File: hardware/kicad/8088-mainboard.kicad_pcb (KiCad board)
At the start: 2 copper layers, 170 x 125 mm, 45 parts, among them J1 Conn_01x10, J2 Exp0, J3 Exp1, J4 POWER 5v, J5 Ext CLK, Q1 NDP6020P, SW1 Reset, SW2 SW_DIP_x02, U1 8088_Min_Mode, U2 74LS373, U3 74LS373, U4 74LS245, U5 8284, U6 74LS138, U7 74LS138, U8 28C256, U9 HM62256BLP, Y1 14.31818 MHz

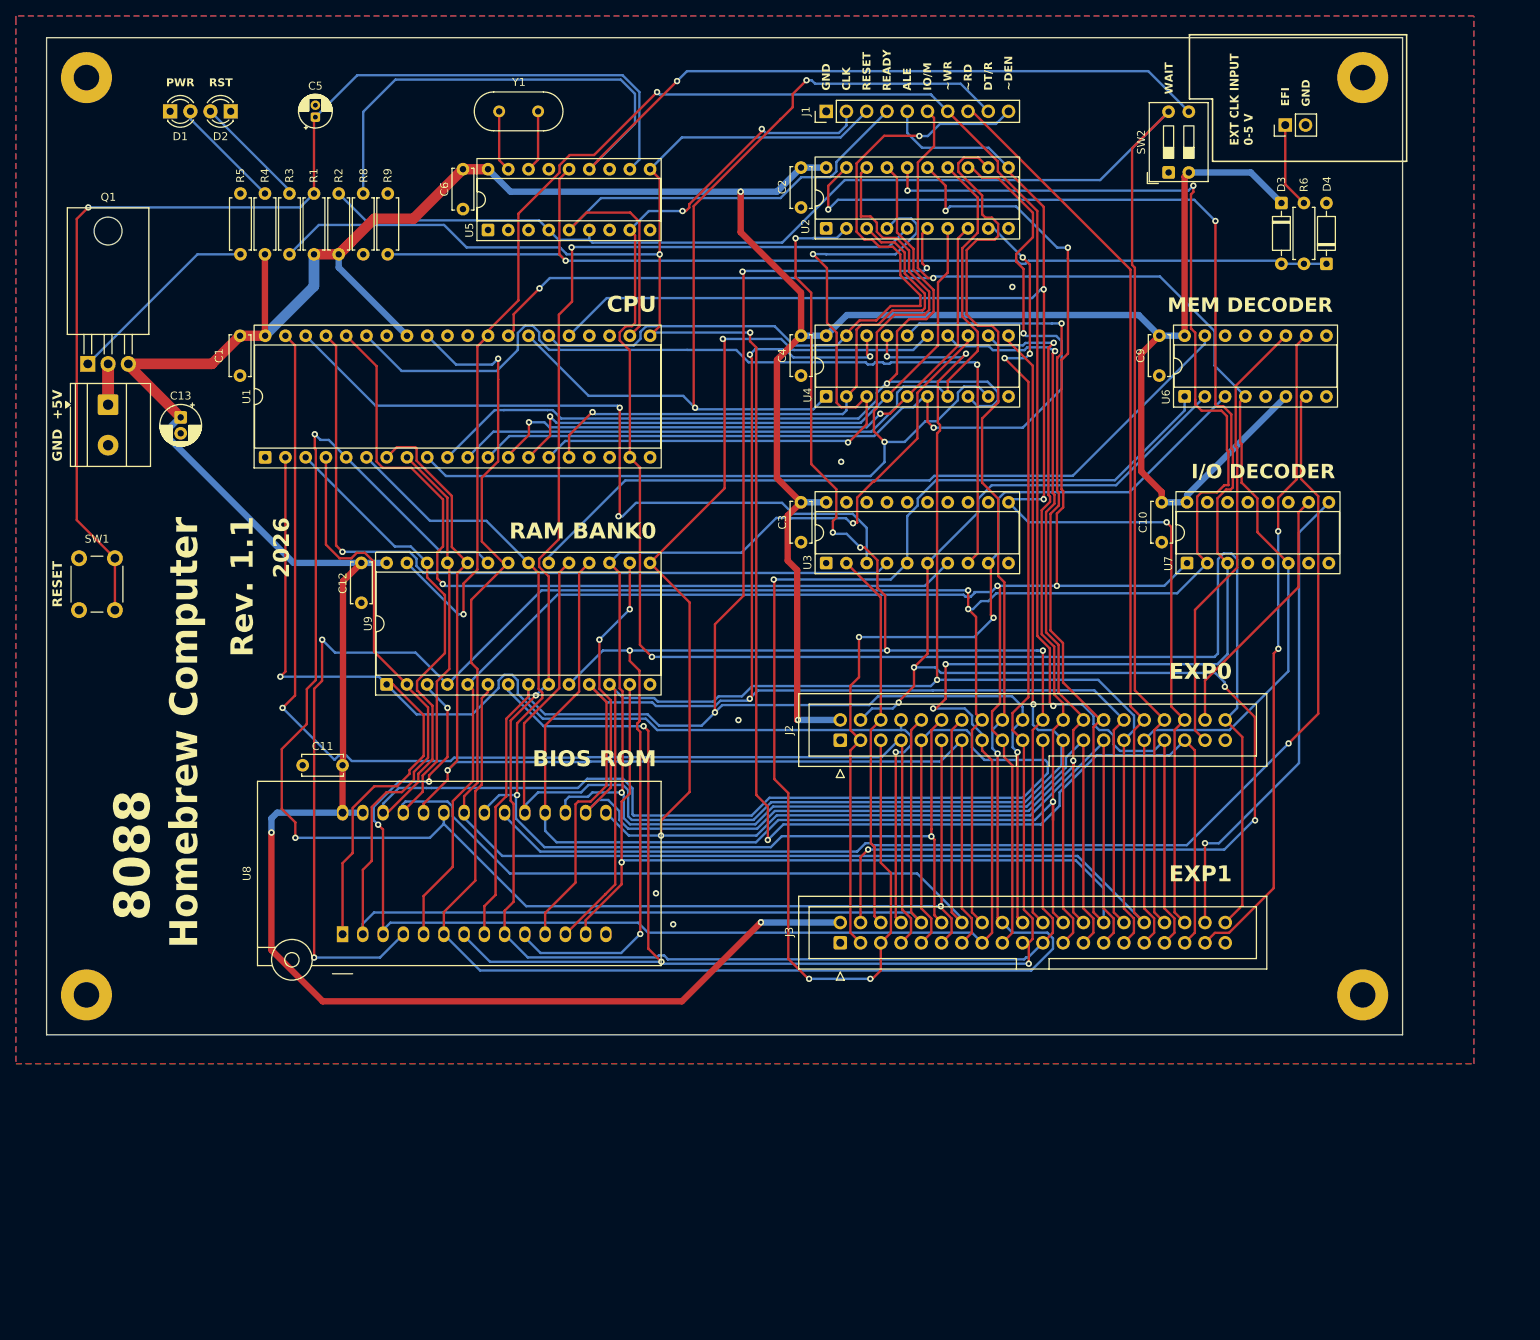
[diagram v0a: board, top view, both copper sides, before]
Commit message: Add mainboard v2.0
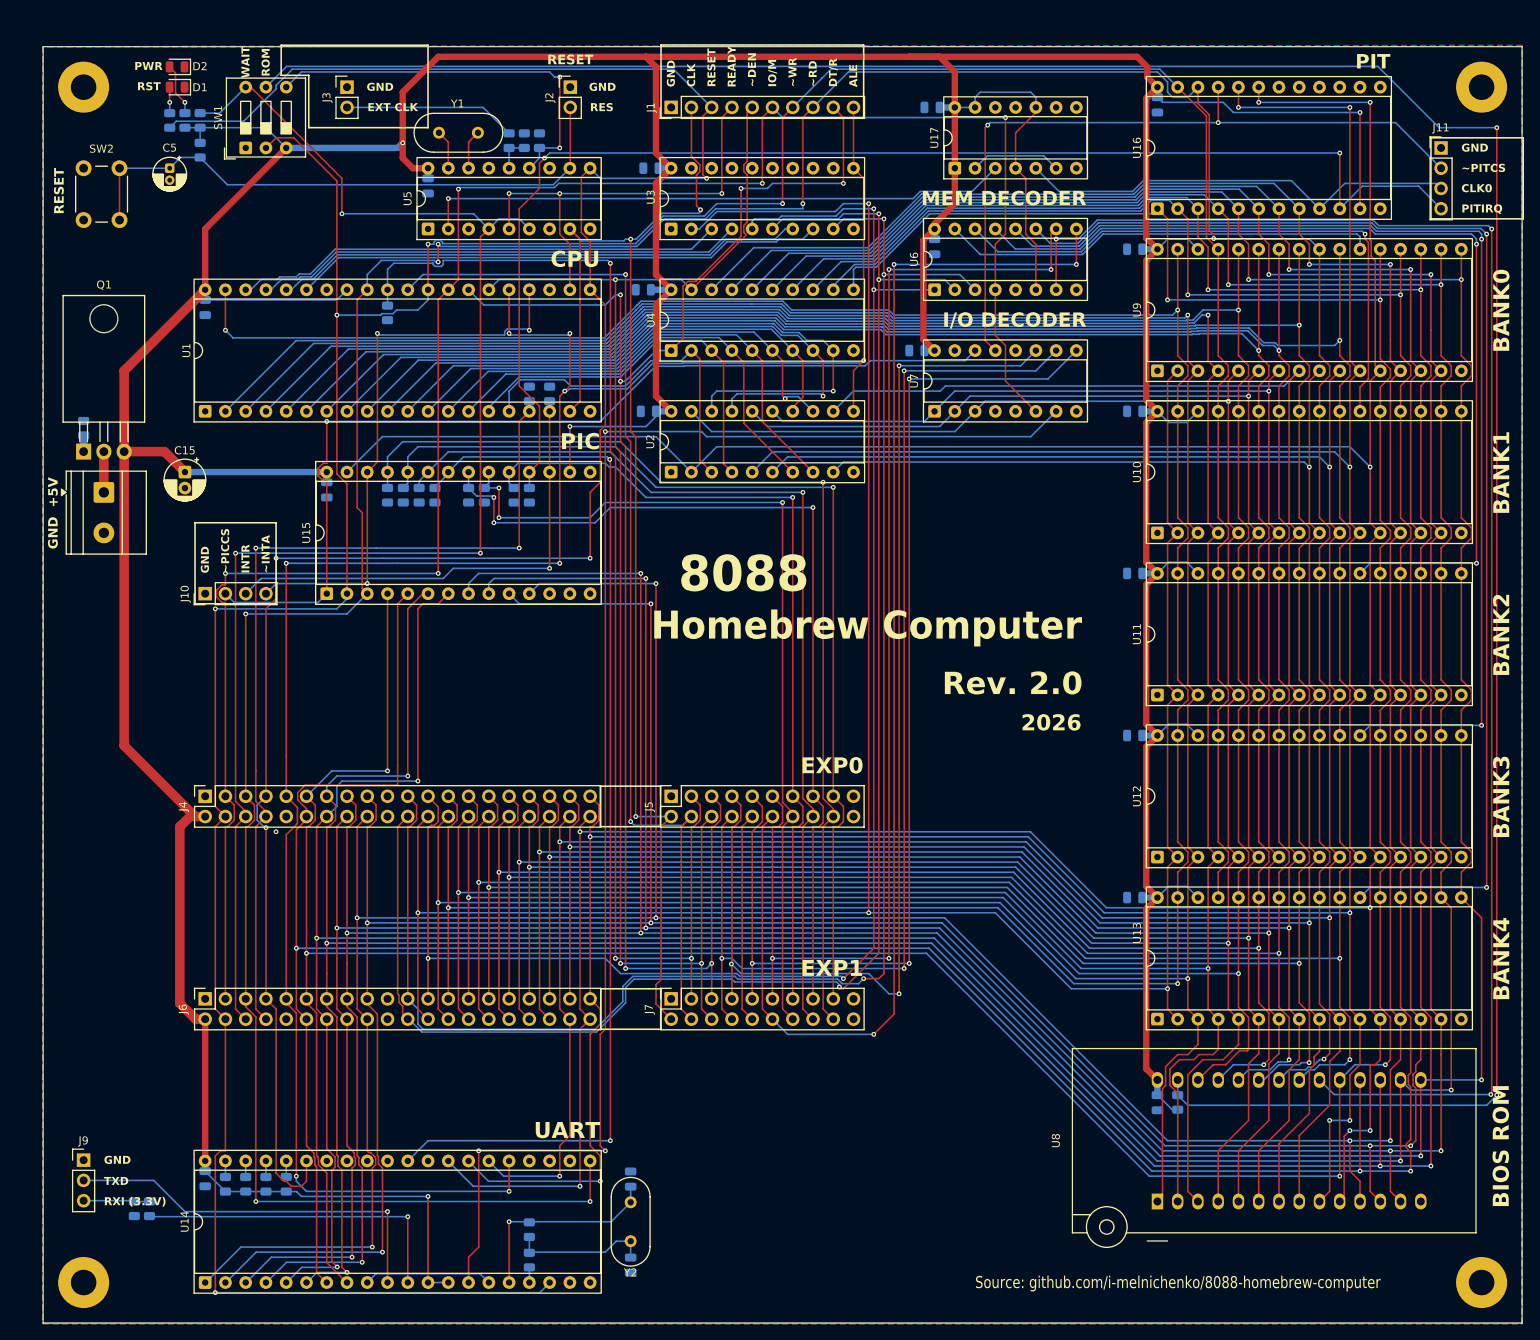
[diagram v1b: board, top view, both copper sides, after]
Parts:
- removed D3, D4: BAT85, Diode_THT:D_DO-35_SOD27_P7.62mm_Horizontal
- removed the J3 at (119.5, 133.5)
- removed the SW2 at (160.7, 36.9)
- added C13: 100nF, Capacitor_SMD:C_0805_2012Metric, B.Cu at (156.4, 107.5)
- added C14: 100nF, Capacitor_SMD:C_0805_2012Metric, B.Cu at (156.4, 127.8)
- added C16: 22pF, Capacitor_SMD:C_0805_2012Metric, B.Cu at (93.2, 163.1)
- added C17: 47pF, Capacitor_SMD:C_0805_2012Metric, B.Cu at (93.2, 173.9)
- added C18: 100nF, Capacitor_SMD:C_0805_2012Metric, B.Cu at (39.9, 163.0)
- added C19: 100nF, Capacitor_SMD:C_0805_2012Metric, B.Cu at (55.1, 76.7)
- added C20: 100nF, Capacitor_SMD:C_0805_2012Metric, B.Cu at (159.3, 28.4)
- added C21: 100nF, Capacitor_SMD:C_0805_2012Metric, B.Cu at (131.0, 28.7)
- added C7: 100nF, Capacitor_SMD:C_0805_2012Metric, B.Cu at (131.3, 46.2)
- added C8: 100nF, Capacitor_SMD:C_0805_2012Metric, B.Cu at (129.1, 59.2)
- added J10: Conn_01x04, Connector_PinHeader_2.54mm:PinHeader_1x04_P2.54mm_Vertical, F.Cu at (39.9, 89.7)
- added J11: Conn_01x04, Connector_PinHeader_2.54mm:PinHeader_1x04_P2.54mm_Vertical, F.Cu at (194.8, 33.8)
- added J4: EXP_0_A, Connector_PinSocket_2.54mm:PinSocket_2x20_P2.54mm_Vertical, F.Cu at (39.9, 115.1)
- added J5: EXP_0_B, Connector_PinSocket_2.54mm:PinSocket_2x10_P2.54mm_Vertical, F.Cu at (98.3, 115.1)
- added J6: EXP_1_A, Connector_PinSocket_2.54mm:PinSocket_2x20_P2.54mm_Vertical, F.Cu at (39.9, 140.5)
- added J7: EXP_1_B, Connector_PinSocket_2.54mm:PinSocket_2x10_P2.54mm_Vertical, F.Cu at (98.3, 140.5)
- added J9: CP2102 Module, Connector_PinHeader_2.54mm:PinHeader_1x03_P2.54mm_Vertical, F.Cu at (24.6, 160.7)
- added R10: 10k, Resistor_SMD:R_0805_2012Metric, B.Cu at (161.8, 153.5)
- added R11: 2k, Resistor_SMD:R_0805_2012Metric, B.Cu at (37.3, 30.4)
- added R12: 10k, Resistor_SMD:R_0805_2012Metric, B.Cu at (24.6, 69.0)
- added R13: 1M, Resistor_SMD:R_0805_2012Metric, B.Cu at (80.5, 169.4)
- added R14: 1.5k, Resistor_SMD:R_0805_2012Metric, B.Cu at (80.5, 173.2)
- added R15: 10k, Resistor_SMD:R_0805_2012Metric, B.Cu at (42.4, 163.7)
- added R16: 10k, Resistor_SMD:R_0805_2012Metric, B.Cu at (45.0, 163.7)
- added R17: 10k, Resistor_SMD:R_0805_2012Metric, B.Cu at (47.5, 163.7)
- added R18: 10k, Resistor_SMD:R_0805_2012Metric, B.Cu at (50.0, 163.7)
- added R19: 1k, Resistor_SMD:R_0805_2012Metric, B.Cu at (32.9, 166.8)
- added R20: 2K, Resistor_SMD:R_0805_2012Metric, B.Cu at (31.0, 166.8)
- added R21: 10k, Resistor_SMD:R_0805_2012Metric, B.Cu at (80.5, 77.4)
- added R22: 10k, Resistor_SMD:R_0805_2012Metric, B.Cu at (78.6, 77.4)
- added R23: 10k, Resistor_SMD:R_0805_2012Metric, B.Cu at (74.9, 77.4)
- added R24: 10k, Resistor_SMD:R_0805_2012Metric, B.Cu at (72.9, 77.4)
- added R25: 10k, Resistor_SMD:R_0805_2012Metric, B.Cu at (68.7, 77.4)
- added R26: 10k, Resistor_SMD:R_0805_2012Metric, B.Cu at (66.7, 77.4)
- added R27: 10k, Resistor_SMD:R_0805_2012Metric, B.Cu at (64.7, 77.4)
- added R28: 10k, Resistor_SMD:R_0805_2012Metric, B.Cu at (62.7, 77.4)
- added R7: 10k, Resistor_SMD:R_0805_2012Metric, B.Cu at (81.8, 32.9)
- added SW1: SW_DIP_x03, Button_Switch_THT:SW_DIP_SPSTx03_Slide_9.78x9.8mm_W7.62mm_P2.54mm, F.Cu at (45.0, 33.8)
- added U10: AS6C1008-55PCN, Package_DIP:DIP-32_W15.24mm_Socket, F.Cu at (159.3, 82.1)
- added U11: AS6C1008-55PCN, Package_DIP:DIP-32_W15.24mm_Socket, F.Cu at (159.3, 102.4)
- added U12: AS6C1008-55PCN, Package_DIP:DIP-32_W15.24mm_Socket, F.Cu at (159.3, 122.7)
- added U13: AS6C1008-55PCN, Package_DIP:DIP-32_W15.24mm_Socket, F.Cu at (159.3, 143.0)
- added U14: GM16C550, Package_DIP:DIP-40_W15.24mm_Socket, F.Cu at (39.9, 176.1)
- added U15: 8259A-2, Package_DIP:DIP-28_W15.24mm_Socket, F.Cu at (55.1, 89.7)
- added U16: 8254, Package_DIP:DIP-24_W15.24mm_Socket, F.Cu at (159.3, 41.4)
- added U17: 74LS74, Package_DIP:DIP-14_W7.62mm_Socket, F.Cu at (133.9, 36.4)
- added Y2: 1.8432 MHz, Crystal:Crystal_HC49-U_Vertical, F.Cu at (93.2, 170.9)
- C1, C10, C11, C12, C2, C3, C4, C6, C9: footprint Capacitor_THT:C_Disc_D5.0mm_W2.5mm_P5.00mm -> Capacitor_SMD:C_0805_2012Metric; moved to B.Cu
- D1: value PWR LED -> RST LED; footprint LED_THT:LED_D3.0mm -> LED_SMD:LED_0805_2012Metric
- D2: value RST LED -> PWR LED; footprint LED_THT:LED_D3.0mm -> LED_SMD:LED_0805_2012Metric
- J2: value Exp0 -> Ext Res; footprint Connector_IDC:IDC-Header_2x20_P2.54mm_Vertical -> Connector_PinHeader_2.54mm:PinHeader_1x02_P2.54mm_Vertical
- R1, R2, R5, R9: footprint Resistor_THT:R_Axial_DIN0207_L6.3mm_D2.5mm_P7.62mm_Horizontal -> Resistor_SMD:R_0805_2012Metric; moved to B.Cu
- R3: value 680 -> 10k; footprint Resistor_THT:R_Axial_DIN0207_L6.3mm_D2.5mm_P7.62mm_Horizontal -> Resistor_SMD:R_0805_2012Metric; moved to B.Cu
- R4: value 2k -> 680; footprint Resistor_THT:R_Axial_DIN0207_L6.3mm_D2.5mm_P7.62mm_Horizontal -> Resistor_SMD:R_0805_2012Metric; moved to B.Cu
- R6: value 1k -> 10k; footprint Resistor_THT:R_Axial_DIN0207_L6.3mm_D2.5mm_P7.62mm_Horizontal -> Resistor_SMD:R_0805_2012Metric; moved to B.Cu
- R8: value 10k -> 1k; footprint Resistor_THT:R_Axial_DIN0207_L6.3mm_D2.5mm_P7.62mm_Horizontal -> Resistor_SMD:R_0805_2012Metric; moved to B.Cu
- U9: value HM62256BLP -> AS6C1008-55PCN; footprint Package_DIP:DIP-28_W15.24mm_Socket -> Package_DIP:DIP-32_W15.24mm_Socket
- moved R6 139.5 mm to (39.2, 30.4)
- moved J3 117.7 mm to (57.7, 26.2), turned to 0 degrees
- moved C11 108.8 mm to (156.4, 66.8)
- moved U8 107.5 mm to (159.3, 165.9)
- moved U9 104.3 mm to (159.3, 61.8)
- moved C12 97.0 mm to (156.4, 87.2), turned to 180 degrees
- moved C9 96.2 mm to (159.3, 153.5)
- moved J2 88.6 mm to (85.7, 26.2), turned to 0 degrees
- moved SW2 48.9 mm to (29.1, 36.4)
- moved U3 46.2 mm to (98.3, 44.0)
- moved C3 45.9 mm to (95.8, 36.4), turned to 180 degrees
- moved H4 39.0 mm to (199.9, 176.1)
- moved U7 36.9 mm to (131.3, 66.8)
- moved U2 36.2 mm to (98.3, 74.5)
- moved H3 36.1 mm to (24.6, 176.1)
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- renumbered C13 to C15, J5 to J3, J4 to J8, SW1 to SW2
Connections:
- net /CPU/DT_R renamed /DT_R
- J1 pad 10: /CPU/DEN -> /ALE
- J1 pad 5: /ALE -> /DEN
- J2 pad 2: VCC -> /CLOCK/RES
- J3 pad 1: Net-(J5-Pin_1) -> GND
- J3 pad 2: GND -> Net-(J3-Pin_2)
- R1 pad 1: VCC -> /HOLD
- R1 pad 2: /CLOCK/RES -> GND
- R2 pad 1: VCC -> /INTR
- R2 pad 2: /RDY -> GND
- R3 pad 1: /RESET -> /NMI
- R3 pad 2: Net-(D2-A) -> GND
- R4 pad 1: VCC -> /RESET
- R5 pad 1: Net-(Q1-G) -> VCC
- R5 pad 2: GND -> /CLOCK/RES
- R6 pad 1: Net-(D3-A) -> VCC
- R6 pad 2: Net-(J5-Pin_1) -> /RDY
- R8 pad 1: Net-(U5-F/~{C}) -> Net-(U5-EFI)
- R8 pad 2: GND -> Net-(J3-Pin_2)
- R9 pad 1: Net-(D3-A) -> Net-(U5-EFI)
- U1 pad 17: GND -> /NMI
- U1 pad 18: GND -> /INTR
- U1 pad 24: unconnected-(U1-~{INTA}-Pad24) -> /INTA
- U1 pad 26: /CPU/DEN -> /DEN
- U1 pad 30: unconnected-(U1-HLDA-Pad30) -> /HLDA
- U1 pad 31: GND -> /HOLD
- U4 pad 19: /CPU/DEN -> /DEN
- U5 pad 13: Net-(U5-F/~{C}) -> /CLOCK_EFI_SW
- U5 pad 14: Net-(D3-A) -> Net-(U5-EFI)
- U5 pad 2: unconnected-(U5-PCLK-Pad2) -> /PCLK
- U6 pad 10: /EXPANSION_CONNECTOR/MEM_EXP1_CS -> /EXP_MEM_CS5
- U6 pad 11: /EXPANSION_CONNECTOR/MEM_EXP0_CS -> /MEM_DECODER/RAM_BANK4_CS
- U6 pad 12: unconnected-(U6-O3-Pad12) -> /MEM_DECODER/RAM_BANK3_CS
- U6 pad 13: unconnected-(U6-O2-Pad13) -> /MEM_DECODER/RAM_BANK2_CS
- U6 pad 14: unconnected-(U6-O1-Pad14) -> /MEM_DECODER/RAM_BANK1_CS
- U6 pad 9: unconnected-(U6-O6-Pad9) -> /EXP_MEM_CS6
- U7 pad 10: /EXPANSION_CONNECTOR/IO_EXP0_CS -> /EXPANSION_CONNECTOR/EXP_IO_CS5
- U7 pad 11: unconnected-(U7-O4-Pad11) -> /EXPANSION_CONNECTOR/EXP_IO_CS4
- U7 pad 13: unconnected-(U7-O2-Pad13) -> /IO_DECODER/IO_PIT_CS
- U7 pad 14: unconnected-(U7-O1-Pad14) -> /IO_DECODER/IO_PIC_CS
- U7 pad 7: unconnected-(U7-O7-Pad7) -> /IO_DECODER/IO_UART_CS
- U7 pad 9: /EXPANSION_CONNECTOR/IO_EXP1_CS -> /EXPANSION_CONNECTOR/EXP_IO_CS6
- U8 pad 27: VCC -> /ROM_WE_SW
- U9 pad 1: /A14 -> unconnected-(U9-NC-Pad1)
- U9 pad 10: /A0 -> /A2
- U9 pad 11: /D0 -> /A1
- U9 pad 12: /D1 -> /A0
- U9 pad 13: /D2 -> /D0
- U9 pad 14: GND -> /D1
- U9 pad 15: /D3 -> /D2
- U9 pad 16: /D4 -> GND
- U9 pad 17: /D5 -> /D3
- U9 pad 18: /D6 -> /D4
- U9 pad 19: /D7 -> /D5
- U9 pad 2: /A12 -> /A16
- U9 pad 20: /MEM_DECODER/RAM_BANK0_CS -> /D6
- U9 pad 21: /A10 -> /D7
- U9 pad 22: /RD -> /MEM_DECODER/RAM_BANK0_CS
- U9 pad 23: /A11 -> /A10
- U9 pad 24: /A9 -> /RD
- U9 pad 25: /A8 -> /A11
- U9 pad 26: /A13 -> /A9
- U9 pad 27: /WR -> /A8
- U9 pad 28: VCC -> /A13
- U9 pad 3: /A7 -> /A14
- U9 pad 4: /A6 -> /A12
- U9 pad 5: /A5 -> /A7
- U9 pad 6: /A4 -> /A6
- U9 pad 7: /A3 -> /A5
- U9 pad 8: /A2 -> /A4
- U9 pad 9: /A1 -> /A3
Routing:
- net /D3: track 191.8 -> 515.1 mm, vias 2 -> 8
- net /ROM_WE_SW: track 0.00 -> 322.8 mm, vias 0 -> 2
- net /D1: track 189.3 -> 502.4 mm, vias 3 -> 8
- net /D2: track 199.8 -> 506.9 mm, vias 2 -> 8
- net /D0: track 195.6 -> 499.4 mm, vias 3 -> 8
- net /D4: track 193.0 -> 476.9 mm, vias 4 -> 7
- net /D6: track 189.0 -> 471.8 mm, vias 2 -> 5
- net /D5: track 194.3 -> 475.1 mm, vias 2 -> 7
- net /A16: track 47.9 -> 322.3 mm, vias 0 -> 4
- net /D7: track 193.9 -> 447.6 mm, vias 1 -> 6
- net /A0: track 214.2 -> 465.4 mm, vias 7 -> 8
- net /A10: track 146.0 -> 388.6 mm, vias 2 -> 4
- net /A9: track 147.4 -> 366.7 mm, vias 1 -> 4
- net VCC: track 540.3 -> 753.1 mm
- net /A8: track 154.2 -> 360.0 mm, vias 0 -> 4
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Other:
- board size 170 x 125 mm -> 185.4 x 160 mm
- board text added: "BANK0"
- board text added: "BANK1"
- board text added: "BANK2"
- board text added: "BANK3"
- board text added: "BANK4"
- board text added: "CLK0"
- board text added: "EXT CLK"
- board text added: "INTR"
- board text added: "PIC"
- board text added: "PIT"
- board text added: "PITIRQ"
- board text added: "RES"
- board text added: "ROM"
- board text added: "RXI (3.3V)"
- board text added: "Rev. 2.0"
- board text added: "TXD"
- board text added: "UART"
- board text added: "~INTA"
- board text added: "~PICCS"
- board text added: "~PITCS"
- board text removed: "EFI"
- board text removed: "EXT CLK INPUT 0-5 V"
- board text removed: "RAM BANK0"
- board text removed: "Rev. 1.1"
